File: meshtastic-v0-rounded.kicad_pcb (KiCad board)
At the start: 2 copper layers, 71 x 46 mm, 88 parts, among them J1 USB_C_Receptacle_USB2.0_16P, J2 Conn_01x02_Pin, J3 Conn_Coaxial, J4 Conn_Coaxial, Q1 SI2302, Q2 Q_PNP_BEC, Q3 Q_NPN_BEC, U1 DM-OLED096-636, U10 LIS3DSHTR, U2 ATGM336H, U3 TPS62046DGQR, U4 HT-RA62, U5 Lever Switch TMHU26, U6 BQ24072RGT, U7 ESP32-S3-WROOM-1, U8 AT24C32A, U9 BME280

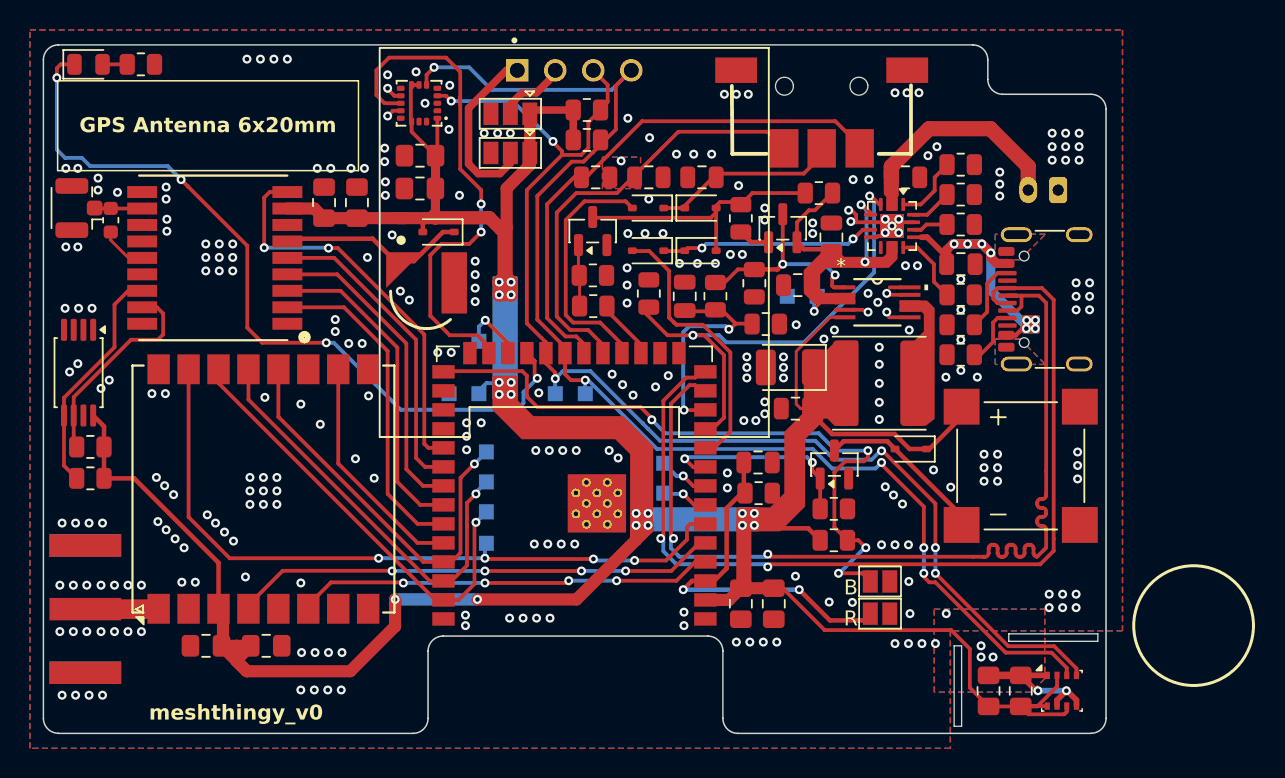
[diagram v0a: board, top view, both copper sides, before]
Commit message: fixed ground clearance, and tidy up
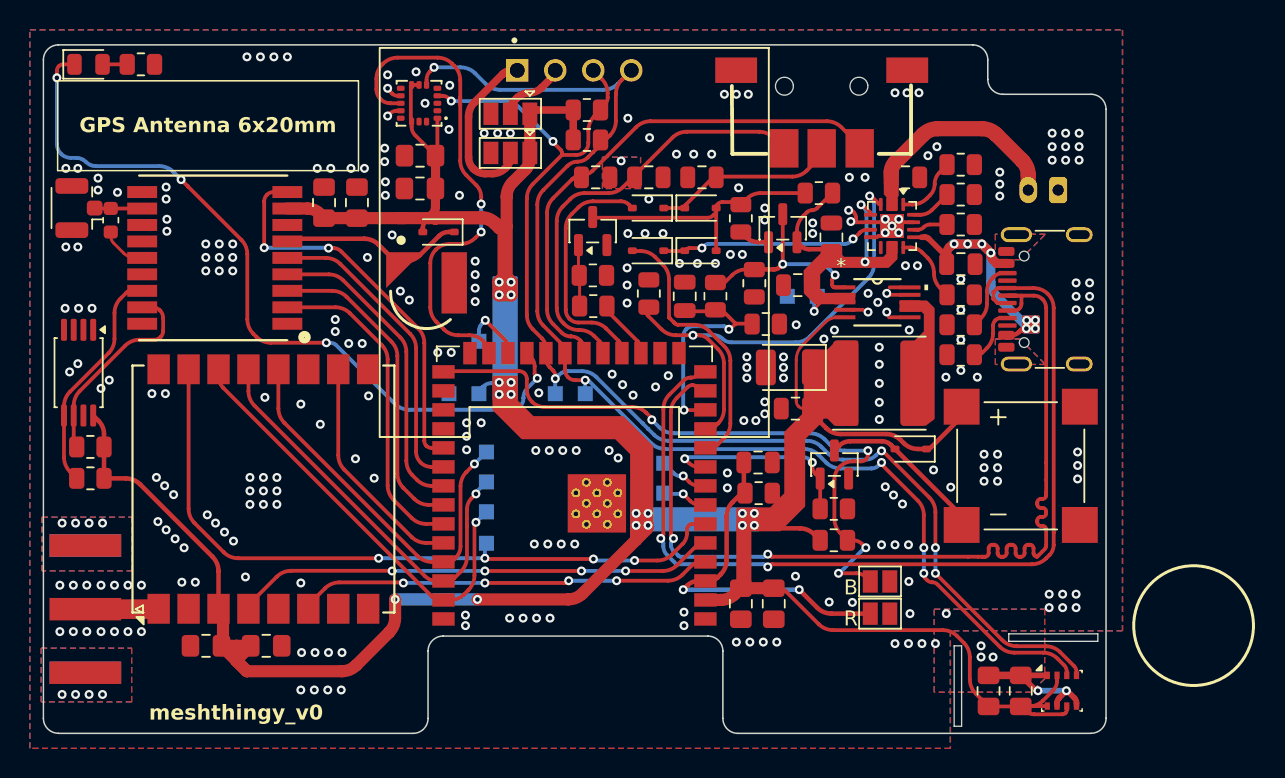
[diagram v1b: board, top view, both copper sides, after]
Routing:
- net +3V3: track 183.2 -> 181.1 mm
- net /Accelerometer/SDA: track 86.1 -> 84.8 mm
- net /Accelerometer/SCL: track 82.8 -> 81.6 mm
- net /Accelerometer/INT: track 34.4 -> 33.5 mm
- net /Connectors/VBUS: track 19.3 -> 18.5 mm
- net /Microcontroller/BOOT: track 45.8 -> 45.0 mm
- net /Microcontroller/STATUS_LED: track 52.5 -> 51.7 mm
- net /Microcontroller/RESET: track 24.8 -> 24.0 mm
- net Net-(D5-A): track 12.4 -> 11.7 mm
- net VSYS: track 16.1 -> 15.4 mm
- net /Microcontroller/PUSH_CCW: track 29.4 -> 28.8 mm
- net /Microcontroller/CHG_EN: track 32.9 -> 32.4 mm
- net /Connectors/D+: track 63.5 -> 63.0 mm
